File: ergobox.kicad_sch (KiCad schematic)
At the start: 14 parts, among them SW1 SW_Push, U1 ATmega32U4-A, Y1 16MHz

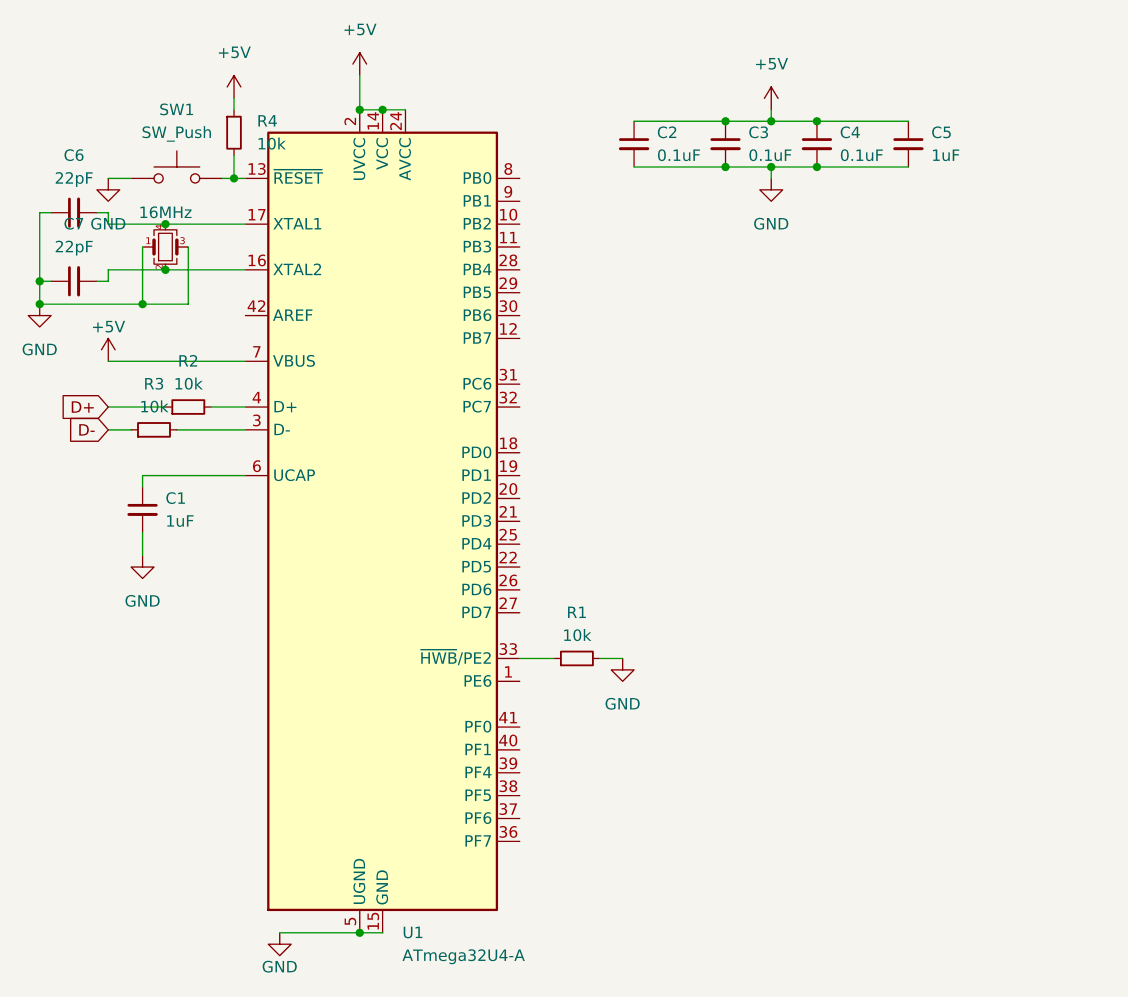
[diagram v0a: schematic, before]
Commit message: add matrix
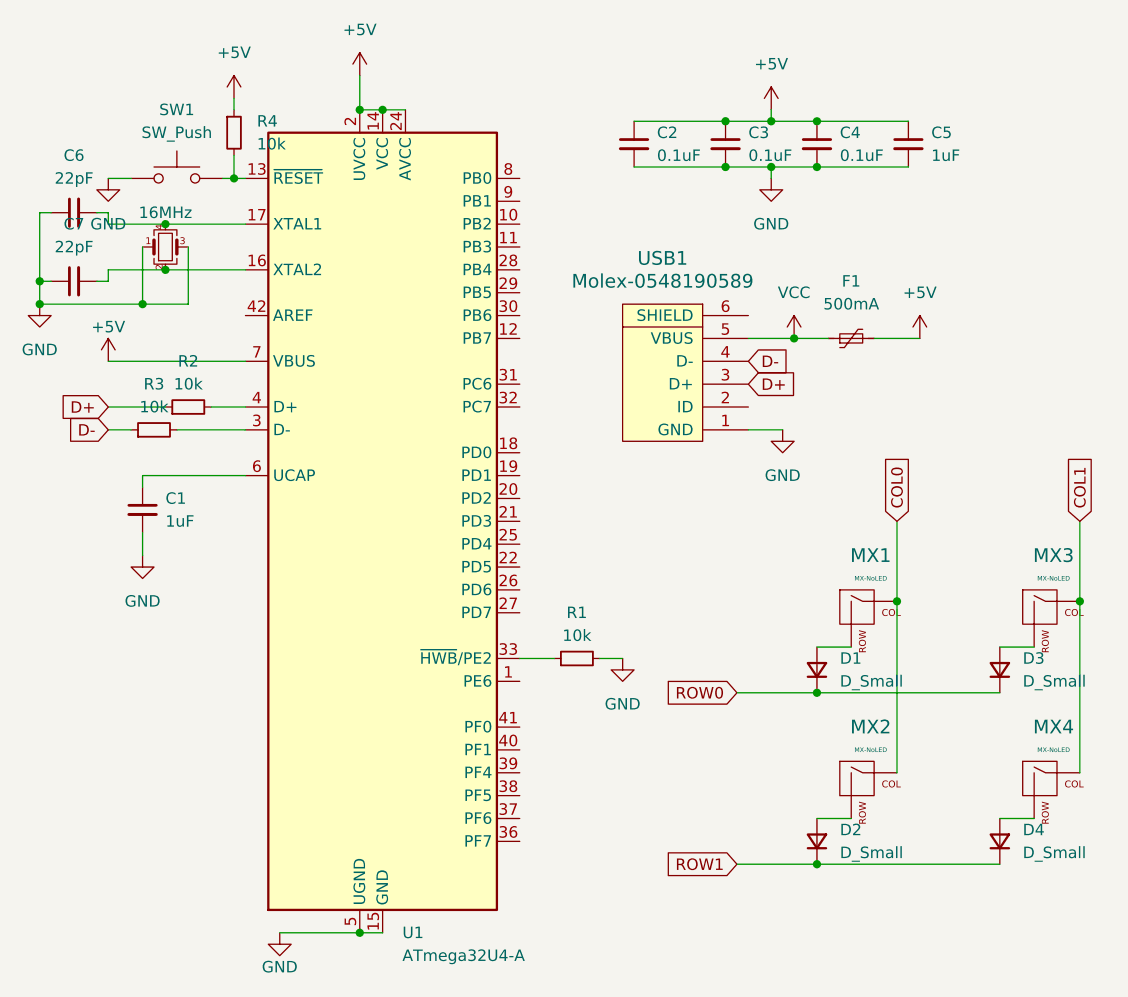
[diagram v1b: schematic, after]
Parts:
- added D1, D2, D3, D4: D_Small, Diode_SMD:D_SOD-123, symbol Device:D_Small
- added F1: 500mA, Fuse:Fuse_1206_3216Metric, symbol Device:Polyfuse_Small
- added MX1, MX2, MX3, MX4: MX-NoLED, MX_Only:MXOnly-1U-NoLED, symbol MX_Alps_Hybrid:MX-NoLED
- added USB1: Molex-0548190589, random-keyboard-parts:Molex-0548190589, symbol random-keyboard-parts:Molex-0548190589
- R1, R2, R3, R4: footprint (none) -> Resistor_SMD:R_0805_2012Metric
- SW1: footprint (none) -> Fuse:Fuse_1206_3216Metric
- Y1: footprint (none) -> Crystal:Crystal_SMD_3225-4Pin_3.2x2.5mm
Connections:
- net +5V: now also F1.2
- net D+: now also USB1.3 (D+)
- net D-: now also USB1.4 (D-)
- net GND: now also USB1.1 (GND)
- new net: D2.2 (A), MX2.2 (ROW)
- new net: D3.2 (A), MX3.2 (ROW)
- new net: D1.2 (A), MX1.2 (ROW)
- new net: D4.2 (A), MX4.2 (ROW)
- new net COL0: MX1.1 (COL), MX2.1 (COL)
- new net COL1: MX3.1 (COL), MX4.1 (COL)
- new net ROW0: D1.1 (K), D3.1 (K)
- new net ROW1: D2.1 (K), D4.1 (K)
- new net VCC: F1.1, USB1.5 (VBUS)
